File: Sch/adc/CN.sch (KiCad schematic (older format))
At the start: 12 parts, among them J1 JP4, J2 Header5, P1 CONN_02X40, U1 LTC2292

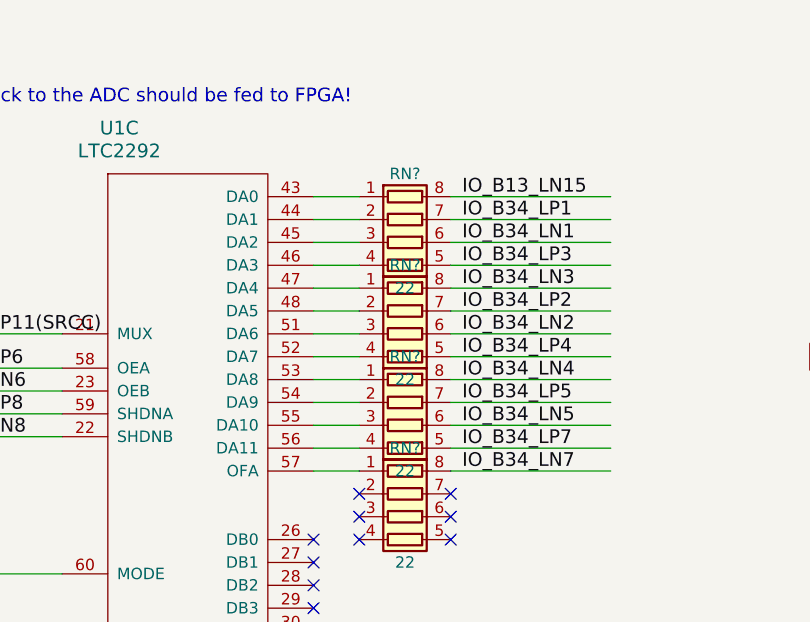
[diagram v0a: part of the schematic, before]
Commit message: Almost finished except Audio
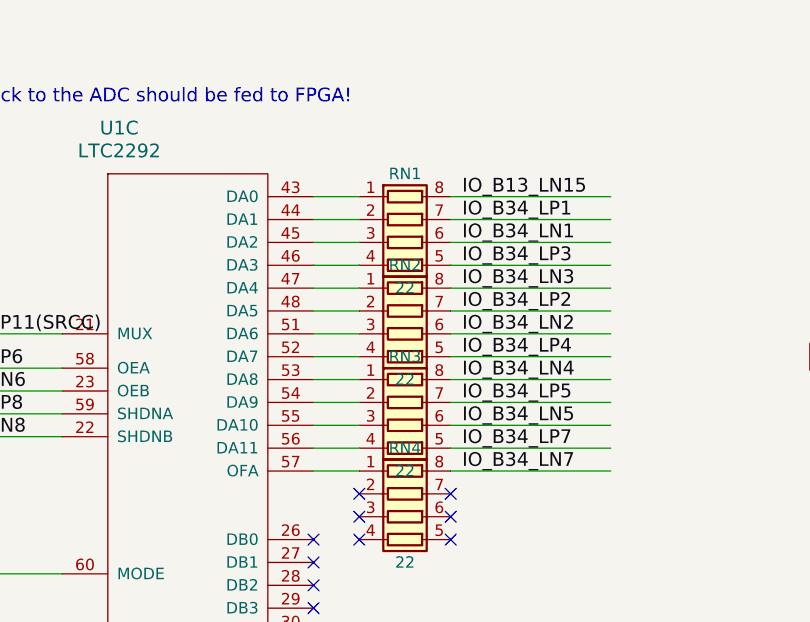
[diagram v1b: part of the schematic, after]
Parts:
- gave numbers to parts that had none: 4
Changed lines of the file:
@@
 NoConn ~ 5950 2250
 $Comp
-L R_Pack04 RN?
+L R_Pack04 RN1
 U 1 1 58A5BF52
 P 3700 2050
-F 0 "RN?" V 3400 2050 50  0000 C CNN
+F 0 "RN1" V 3400 2050 50  0000 C CNN
 F 1 "22" V 3900 2050 50  0000 C CNN
 F 2 "" V 3975 2050 50  0001 C CNN
@@
 $EndComp
 $Comp
-L R_Pack04 RN?
+L R_Pack04 RN2
 U 1 1 58A5BFD7
 P 3700 2450
-F 0 "RN?" V 3400 2450 50  0000 C CNN
+F 0 "RN2" V 3400 2450 50  0000 C CNN
 F 1 "22" V 3900 2450 50  0000 C CNN
 F 2 "" V 3975 2450 50  0001 C CNN
@@
 $EndComp
 $Comp
-L R_Pack04 RN?
+L R_Pack04 RN3
 U 1 1 58A5C027
 P 3700 2850
-F 0 "RN?" V 3400 2850 50  0000 C CNN
+F 0 "RN3" V 3400 2850 50  0000 C CNN
 F 1 "22" V 3900 2850 50  0000 C CNN
 F 2 "" V 3975 2850 50  0001 C CNN
@@
 $EndComp
 $Comp
-L R_Pack04 RN?
+L R_Pack04 RN4
 U 1 1 58A5C02D
 P 3700 3250
-F 0 "RN?" V 3400 3250 50  0000 C CNN
+F 0 "RN4" V 3400 3250 50  0000 C CNN
 F 1 "22" V 3900 3250 50  0000 C CNN
 F 2 "" V 3975 3250 50  0001 C CNN
